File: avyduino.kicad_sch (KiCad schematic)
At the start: 4 parts, among them J1 Power, J2 Digital/PWM, J3 Analog, J4 Digital/PWM

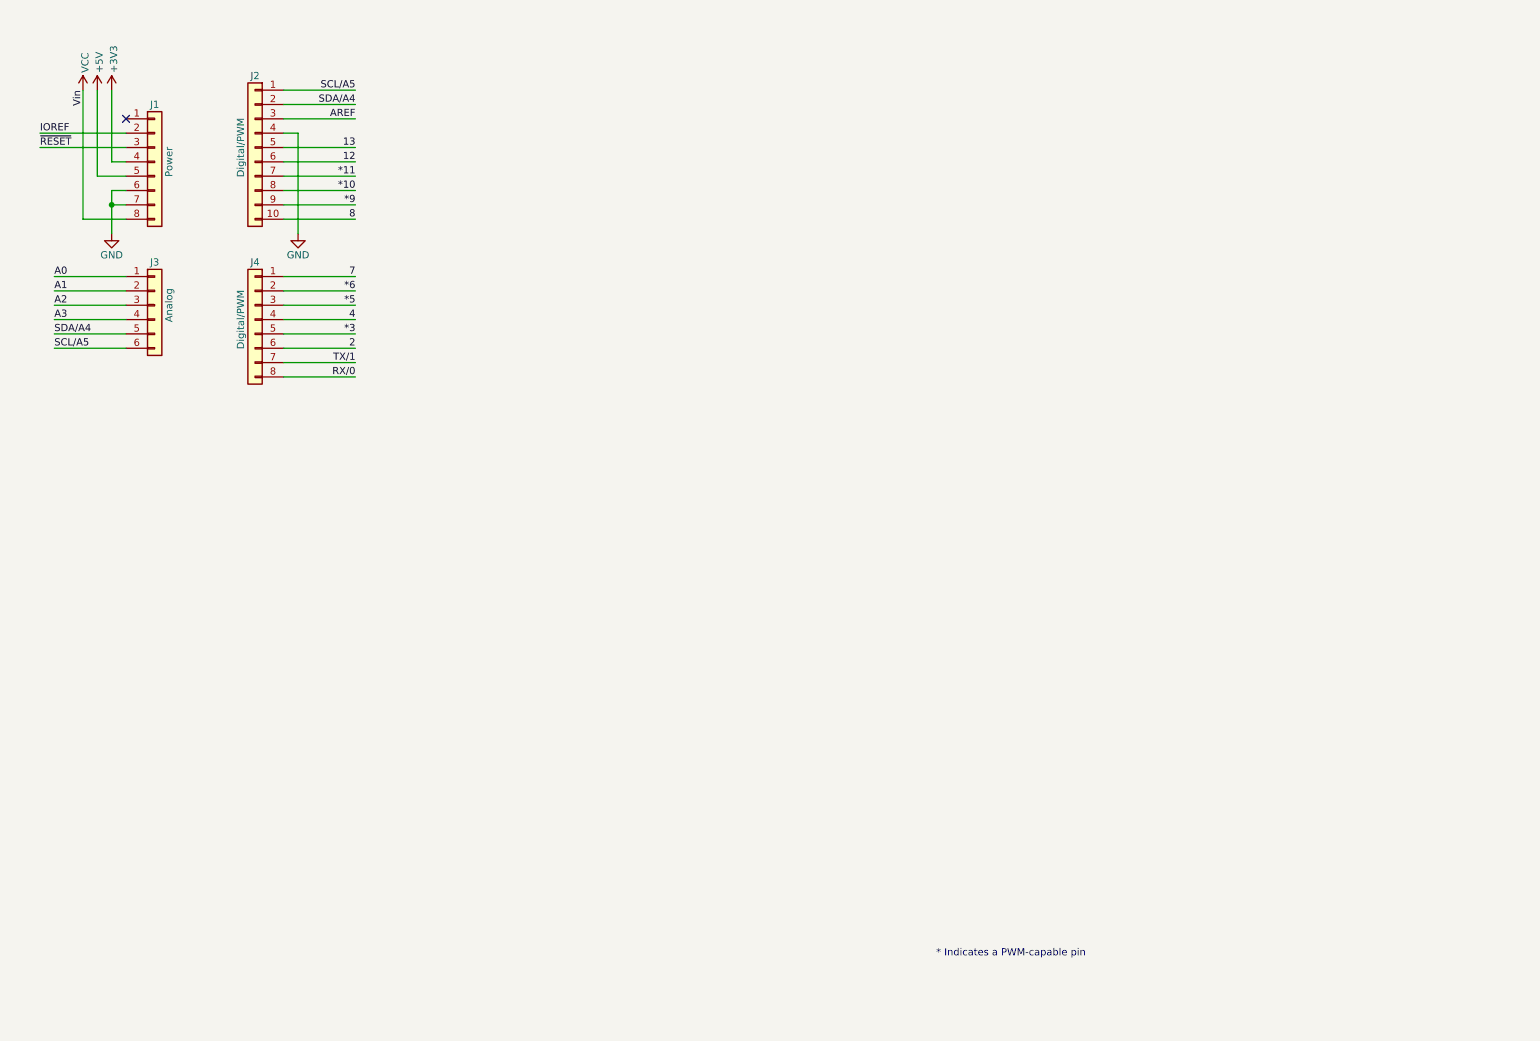
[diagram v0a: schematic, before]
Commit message: make schematic
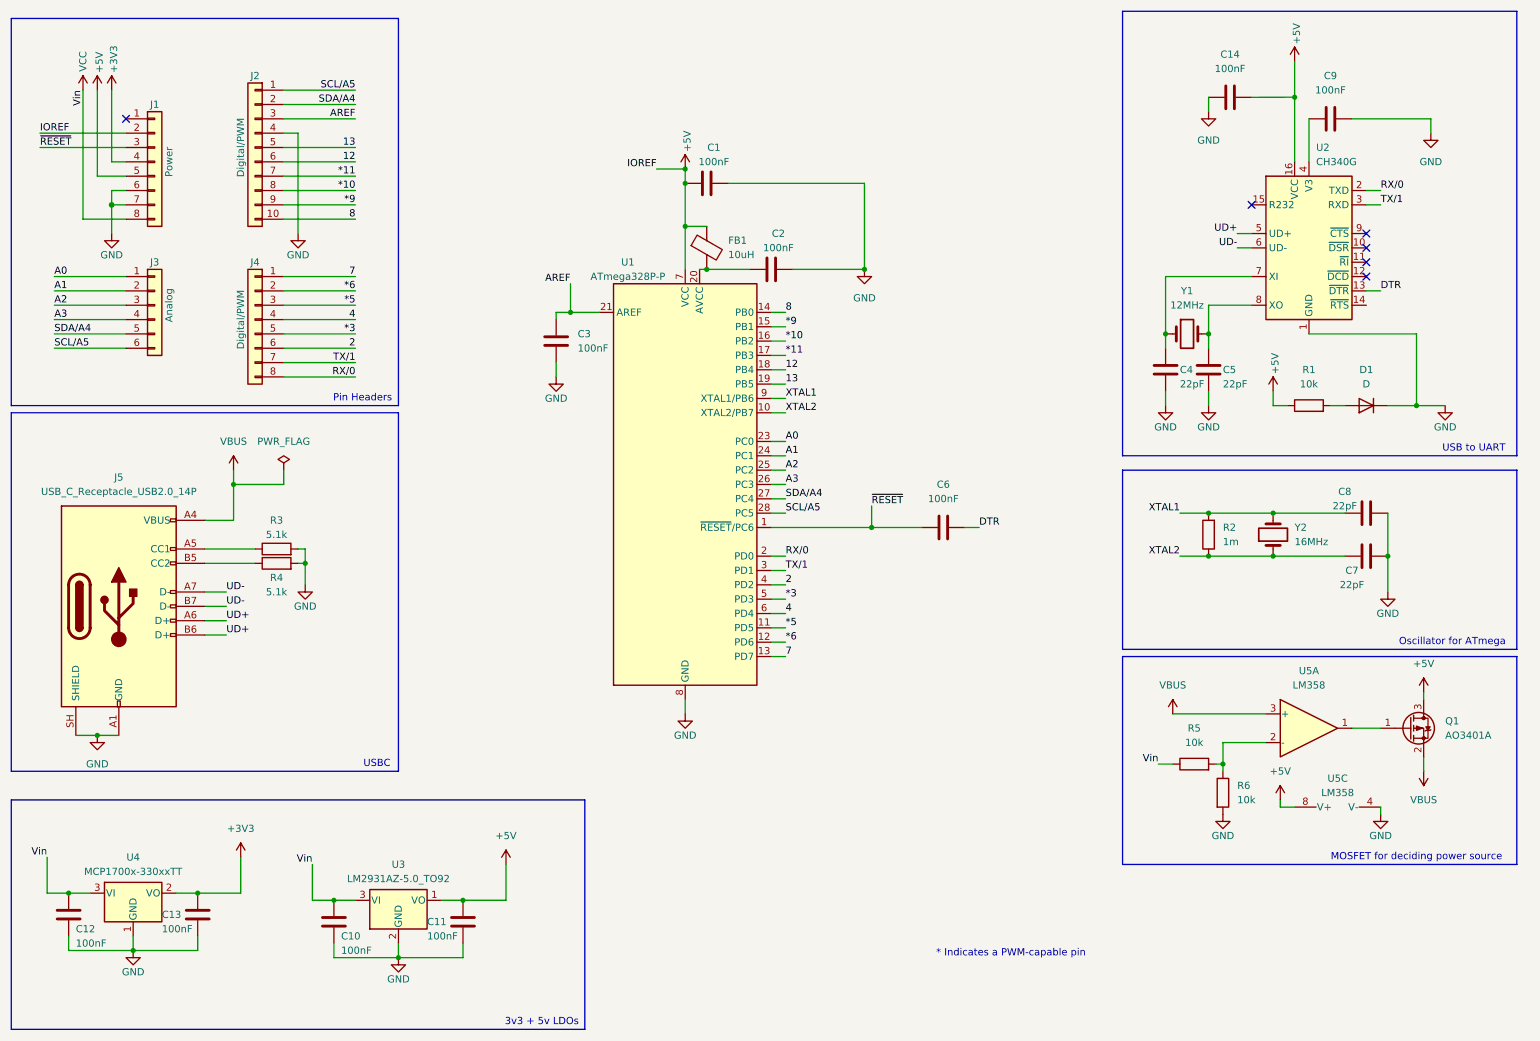
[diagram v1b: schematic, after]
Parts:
- added C1, C10, C11, C12, C13, C14, C2, C3, C6, C9: 100nF, symbol Device:C
- added C4, C5, C7, C8: 22pF, symbol Device:C
- added D1: D, symbol Device:D
- added FB1: 10uH, symbol Device:FerriteBead
- added J5: USB_C_Receptacle_USB2.0_14P, symbol Connector:USB_C_Receptacle_USB2.0_14P
- added Q1: AO3401A, Package_TO_SOT_SMD:SOT-23, symbol Transistor_FET:AO3401A
- added R1, R5, R6: 10k, symbol Device:R
- added R2: 1m, symbol Device:R
- added R3, R4: 5.1k, symbol Device:R
- added U1: ATmega328P-P, Package_DIP:DIP-28_W7.62mm_Socket_LongPads, symbol MCU_Microchip_ATmega:ATmega328P-P
- added U2: CH340G, Package_SO:SOIC-16_3.9x9.9mm_P1.27mm, symbol Interface_USB:CH340G
- added U3: LM2931AZ-5.0_TO92, Package_TO_SOT_THT:TO-92_Inline, symbol Regulator_Linear:LM2931AZ-5.0_TO92
- added U4: MCP1700x-330xxTT, Package_TO_SOT_SMD:SOT-23, symbol Regulator_Linear:MCP1700x-330xxTT
- added U5: LM358, symbol Amplifier_Operational:LM358
- added Y1: 12MHz, symbol Device:Crystal
- added Y2: 16MHz, symbol Device:Crystal
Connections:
- net IOREF is gone; now on net +5V: J1.2 (Pin_2)
- net *10: now also U1.16 (PB2)
- net *11: now also U1.17 (PB3)
- net *3: now also U1.5 (PD3)
- net *5: now also U1.11 (PD5)
- net *6: now also U1.12 (PD6)
- net *9: now also U1.15 (PB1)
- net +3V3: now also C13.2, U4.2 (VO)
- net +5V: now also C1.1, C11.2, C14.2, FB1.1, Q1.3 (D), R1.1, U1.7 (VCC), U2.16 (VCC), U3.1 (VO), U5.8 (V+)
- net 12: now also U1.18 (PB4)
- net 13: now also U1.19 (PB5)
- net 2: now also U1.4 (PD2)
- net 4: now also U1.6 (PD4)
- net 7: now also U1.13 (PD7)
- net 8: now also U1.14 (PB0)
- net A0: now also U1.23 (PC0)
- net A1: now also U1.24 (PC1)
- net A2: now also U1.25 (PC2)
- net A3: now also U1.26 (PC3)
- net AREF: now also C3.1, U1.21 (AREF)
- net GND: now also C1.2, C10.1, C11.1, C12.1, C13.1, C14.1, C2.2, C3.2, C4.2, C5.2, C7.2, C8.2, C9.2, D1.1 (K), J5.A1 (GND), J5.A12 (GND), J5.B1 (GND), J5.B12 (GND), J5.SH (SHIELD), R3.2, R4.2, R6.2, U1.22 (GND), U1.8 (GND), U2.1 (GND), U3.2 (GND), U4.1 (GND), U5.4 (V-)
- net RX/0: now also U1.2 (PD0), U2.2 (TXD)
- net SCL/A5: now also U1.28 (PC5)
- net SDA/A4: now also U1.27 (PC4)
- net TX/1: now also U1.3 (PD1), U2.3 (RXD)
- net VCC: now also C10.2, C12.2, R5.1, U3.3 (VI), U4.3 (VI)
- net ~{RESET}: now also C6.1, U1.1 (~{RESET}/PC6)
- new net: Q1.1 (G), U5.1
- new net: R5.2, R6.1, U5.2 (-)
- new net: J5.A5 (CC1), R3.1
- new net: C4.1, U2.7 (XI), Y1.1
- new net: C5.1, U2.8 (XO), Y1.2
- new net: C9.1, U2.4 (V3)
- new net: C2.1, FB1.2, U1.20 (AVCC)
- new net: D1.2 (A), R1.2
- new net: J5.B5 (CC2), R4.1
- new net DTR: C6.2, U2.13 (~{DTR})
- new net UD+: J5.A6 (D+), J5.B6 (D+), U2.5 (UD+)
- new net UD-: J5.A7 (D-), J5.B7 (D-), U2.6 (UD-)
- new net VBUS: J5.A4 (VBUS), J5.A9 (VBUS), J5.B4 (VBUS), J5.B9 (VBUS), Q1.2 (S), U5.3 (+)
- new net XTAL1: C8.1, R2.2, U1.9 (XTAL1/PB6), Y2.2
- new net XTAL2: C7.1, R2.1, U1.10 (XTAL2/PB7), Y2.1
- no-connect marks 1 -> 6
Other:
- note added: "3v3 + 5v LDOs"
- note added: "MOSFET for deciding power source"
- note added: "Oscillator for ATmega"
- note added: "Pin Headers"
- note added: "USB to UART"
- note added: "USBC"

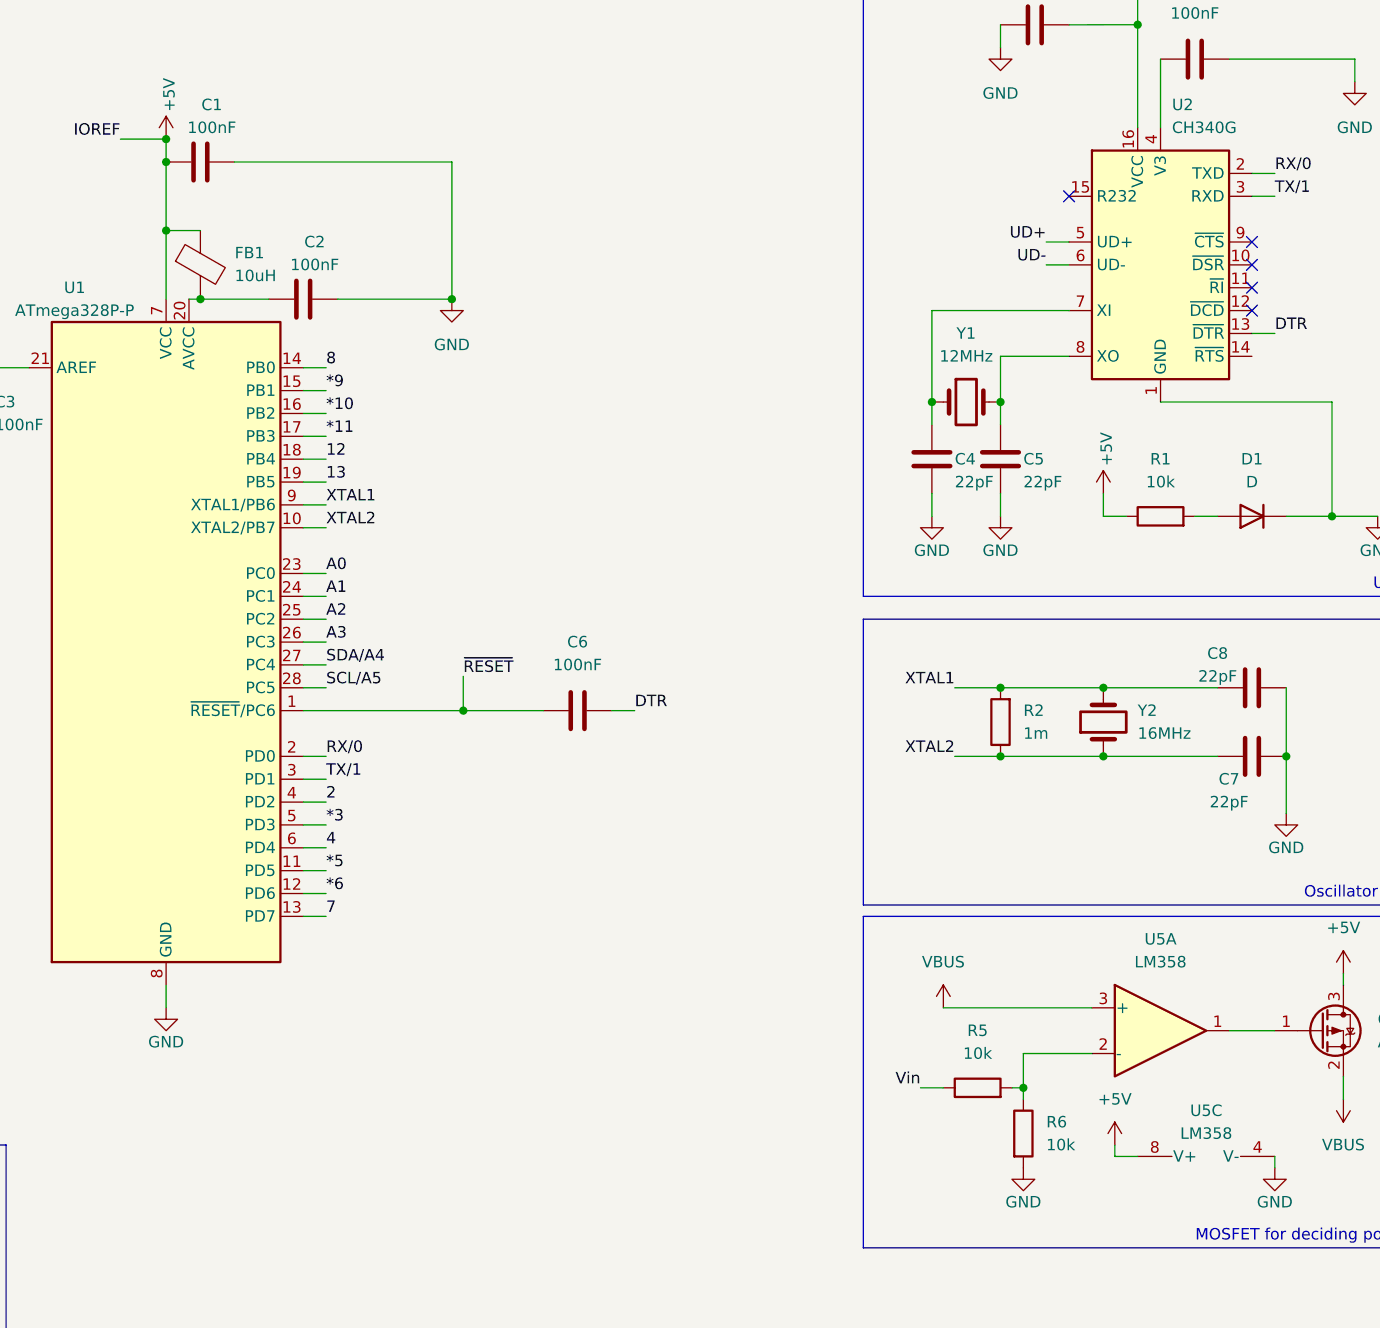
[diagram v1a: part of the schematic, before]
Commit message: do layout
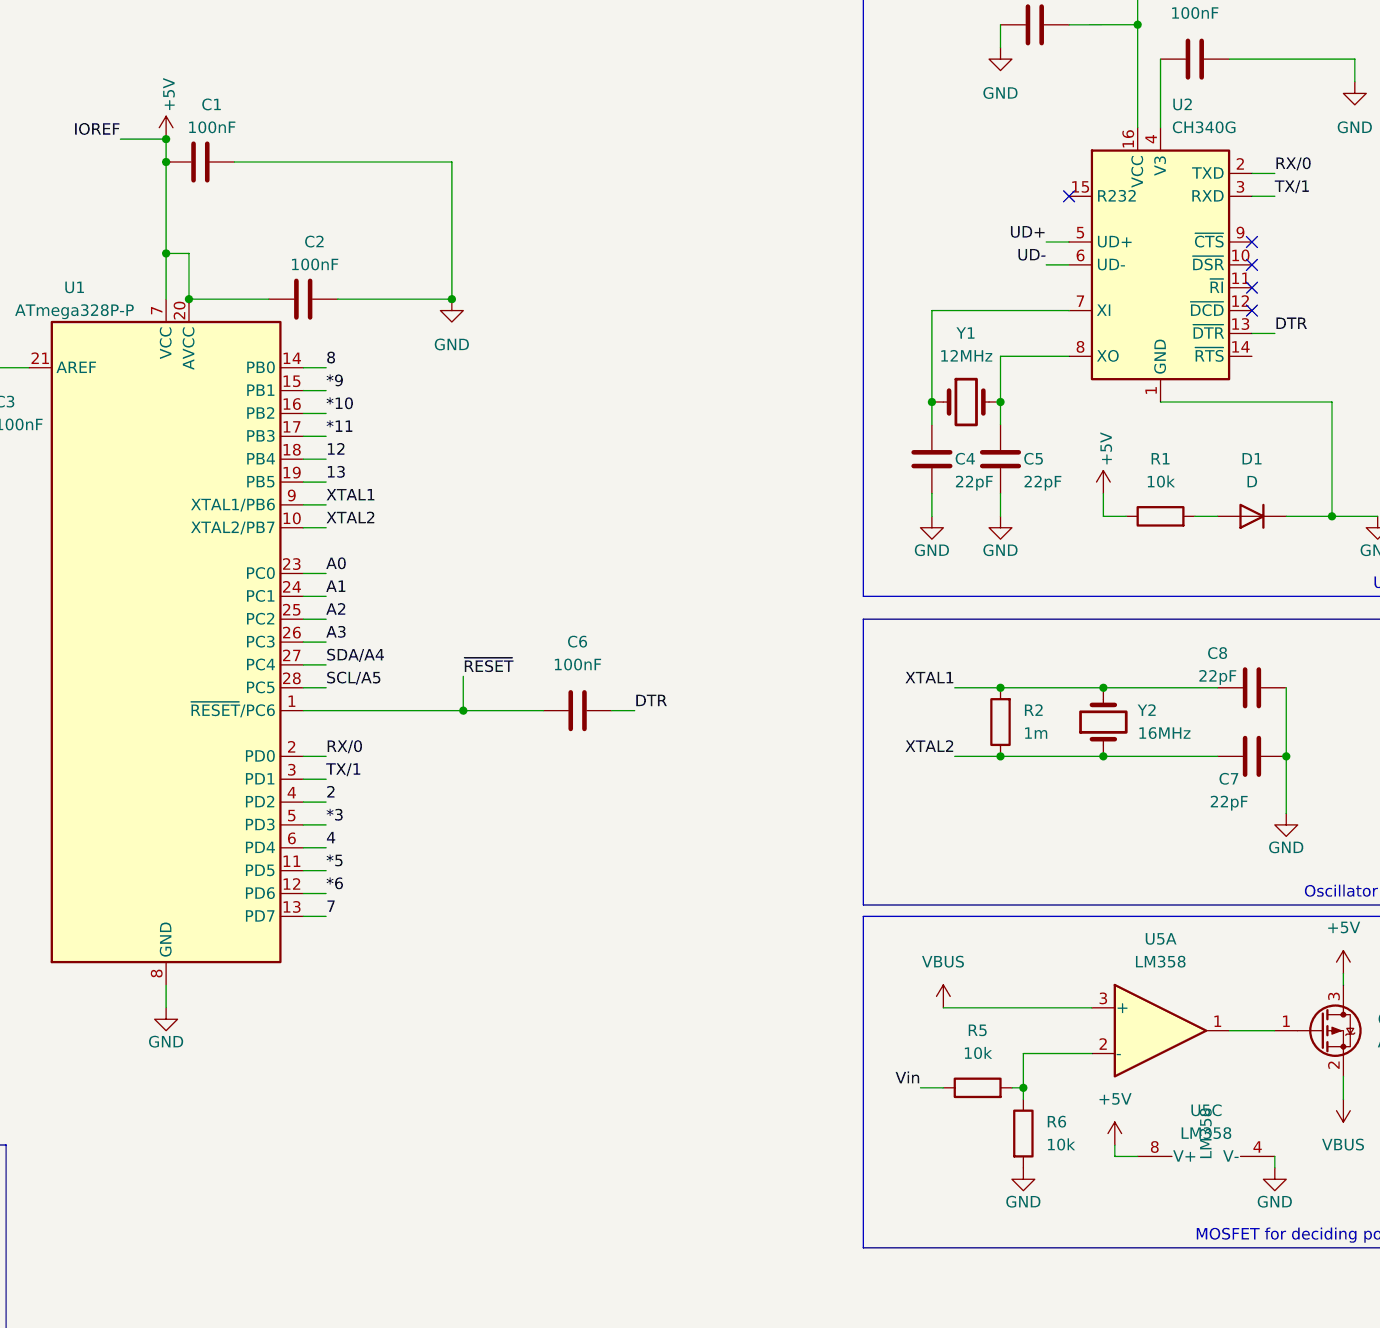
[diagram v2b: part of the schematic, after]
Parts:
- removed FB1: 10uH, symbol Device:FerriteBead
- C1, C10, C11, C12, C13, C14, C2, C3, C4, C5, C6, C7, C8, C9: footprint (none) -> Capacitor_SMD:C_0805_2012Metric
- D1: footprint (none) -> Diode_THT:D_DO-35_SOD27_P10.16mm_Horizontal
- J5: footprint (none) -> Connector_USB:USB_C_Receptacle_GCT_USB4105-xx-A_16P_TopMnt_Horizontal
- Q1: MPN (none) -> AO3401A
- R1, R2, R3, R4, R5, R6: footprint (none) -> Resistor_SMD:R_0805_2012Metric
- U1: MPN (none) -> ATmega328P-P
- U2: MPN (none) -> CH340G
- U3: MPN (none) -> LM2931AZ-5.0_TO92
- U4: MPN (none) -> MCP1700x-330xxTT
- U5: footprint (none) -> Package_DIP:DIP-8_W7.62mm_Socket_LongPads; MPN (none) -> LM358
- Y1, Y2: footprint (none) -> Crystal:Crystal_HC49-U_Vertical
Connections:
- net +5V: now also C2.1, U1.20 (AVCC)
